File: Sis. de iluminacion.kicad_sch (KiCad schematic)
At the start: 48 parts, among them J1 Screw_Terminal_01x02, J10 Screw_Terminal_01x02, J11 Screw_Terminal_01x02, J12 Screw_Terminal_01x02, J3 Screw_Terminal_01x02, J4 Conn_01x04, J5 Screw_Terminal_01x02, J7 Screw_Terminal_01x02, J8 Screw_Terminal_01x02, J9 Screw_Terminal_01x02, K10 Relay_DPDT, K11 Relay_DPDT, K8 Relay_DPDT, K9 Relay_DPDT, Q4 BC547, Q5 BC547, Q6 BC547, Q7 BC547, U1 ESP32_DEVKITC, U10 PC817, U11 PC817, U12 PC817, U13 PC817, U3 L7805

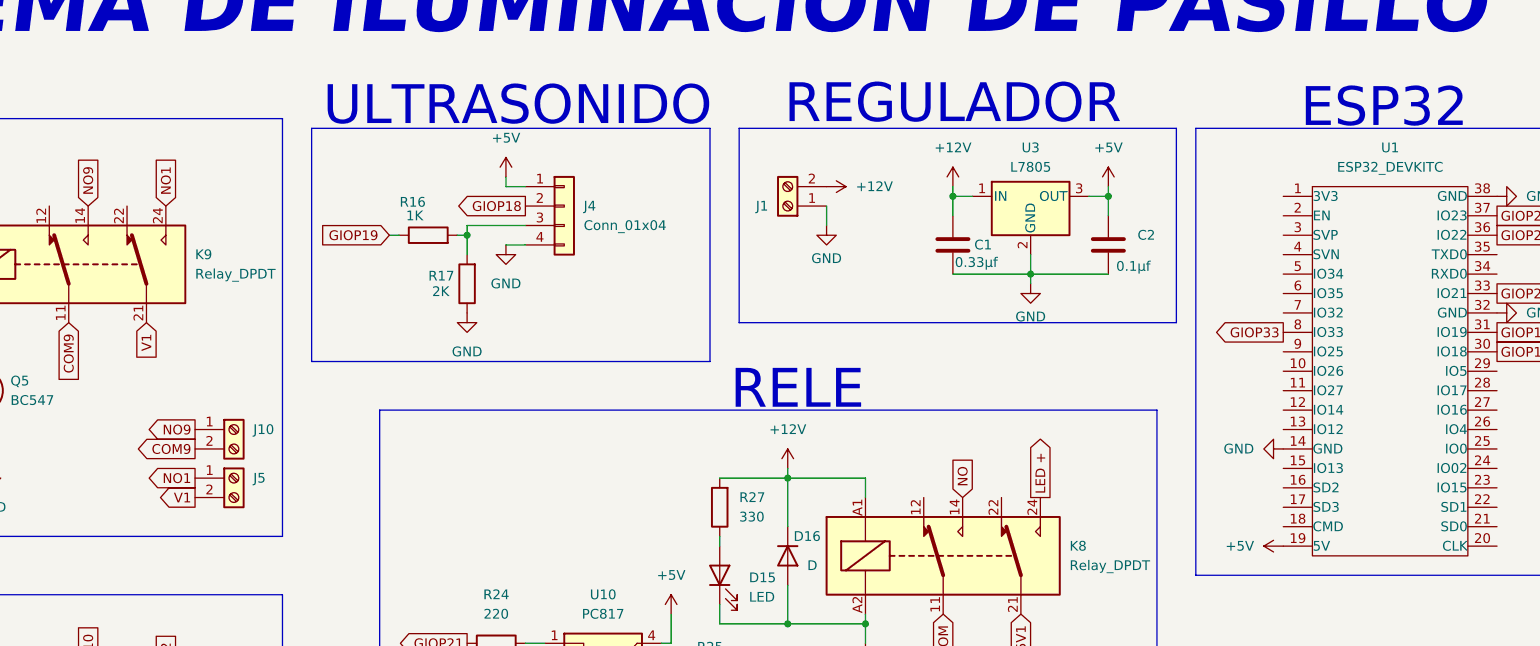
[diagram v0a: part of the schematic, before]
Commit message: Add files via upload
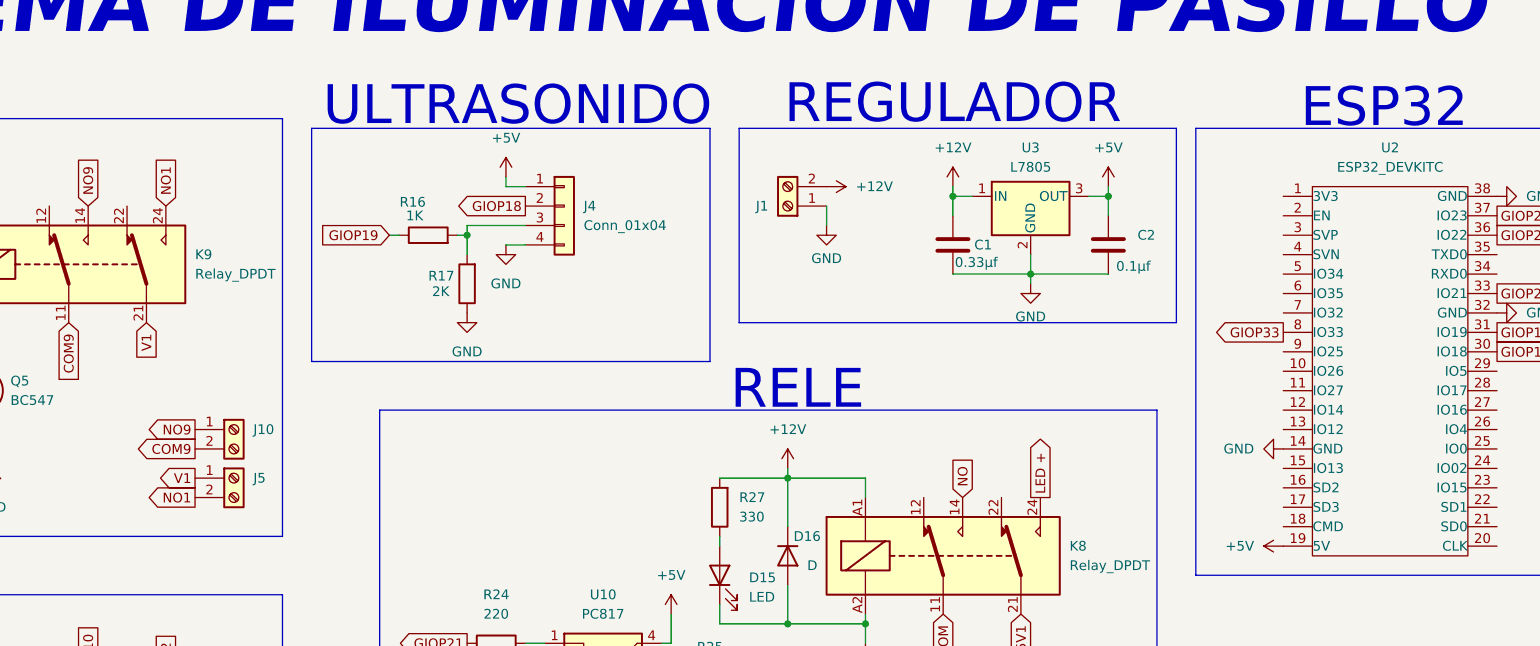
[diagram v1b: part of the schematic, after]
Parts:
- removed U1: ESP32_DEVKITC, EESTN5:ESP32_DEVKITC, symbol EESTN5:ESP32_DEVKITC
- added U2: ESP32_DEVKITC, EESTN5:ESP32S, symbol EESTN5:ESP32_DEVKITC
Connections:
- net +5V: now also U2.19 (5V)
- net GIOP18: now also U2.30 (IO18)
- net GIOP19: now also U2.31 (IO19)
- net GIOP21: now also U2.33 (IO21)
- net GIOP22: now also U2.36 (IO22)
- net GIOP23: now also U2.37 (IO23)
- net GIOP33: now also U2.8 (IO33)
- net GND: now also U2.14 (GND), U2.32 (GND), U2.38 (GND)
- net NO1: now also J5.2 (Pin_2); no longer J5.1 (Pin_1)
- net V1: now also J5.1 (Pin_1); no longer J5.2 (Pin_2)
